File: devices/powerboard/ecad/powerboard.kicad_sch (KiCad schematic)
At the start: 42 parts, among them J1 Conn_02x02_Top_Bottom, J10 Conn_02x01, J2 Conn_02x02_Top_Bottom, J3 Conn_02x01, J4 Conn_02x01, J5 USB_A, J6 JST PH, J7 JST PH, J8 47053-1000, J9 USB_A, Q2 MMBT3904, U1 TPS51386RJNR, U2 EMC2101-ACZL

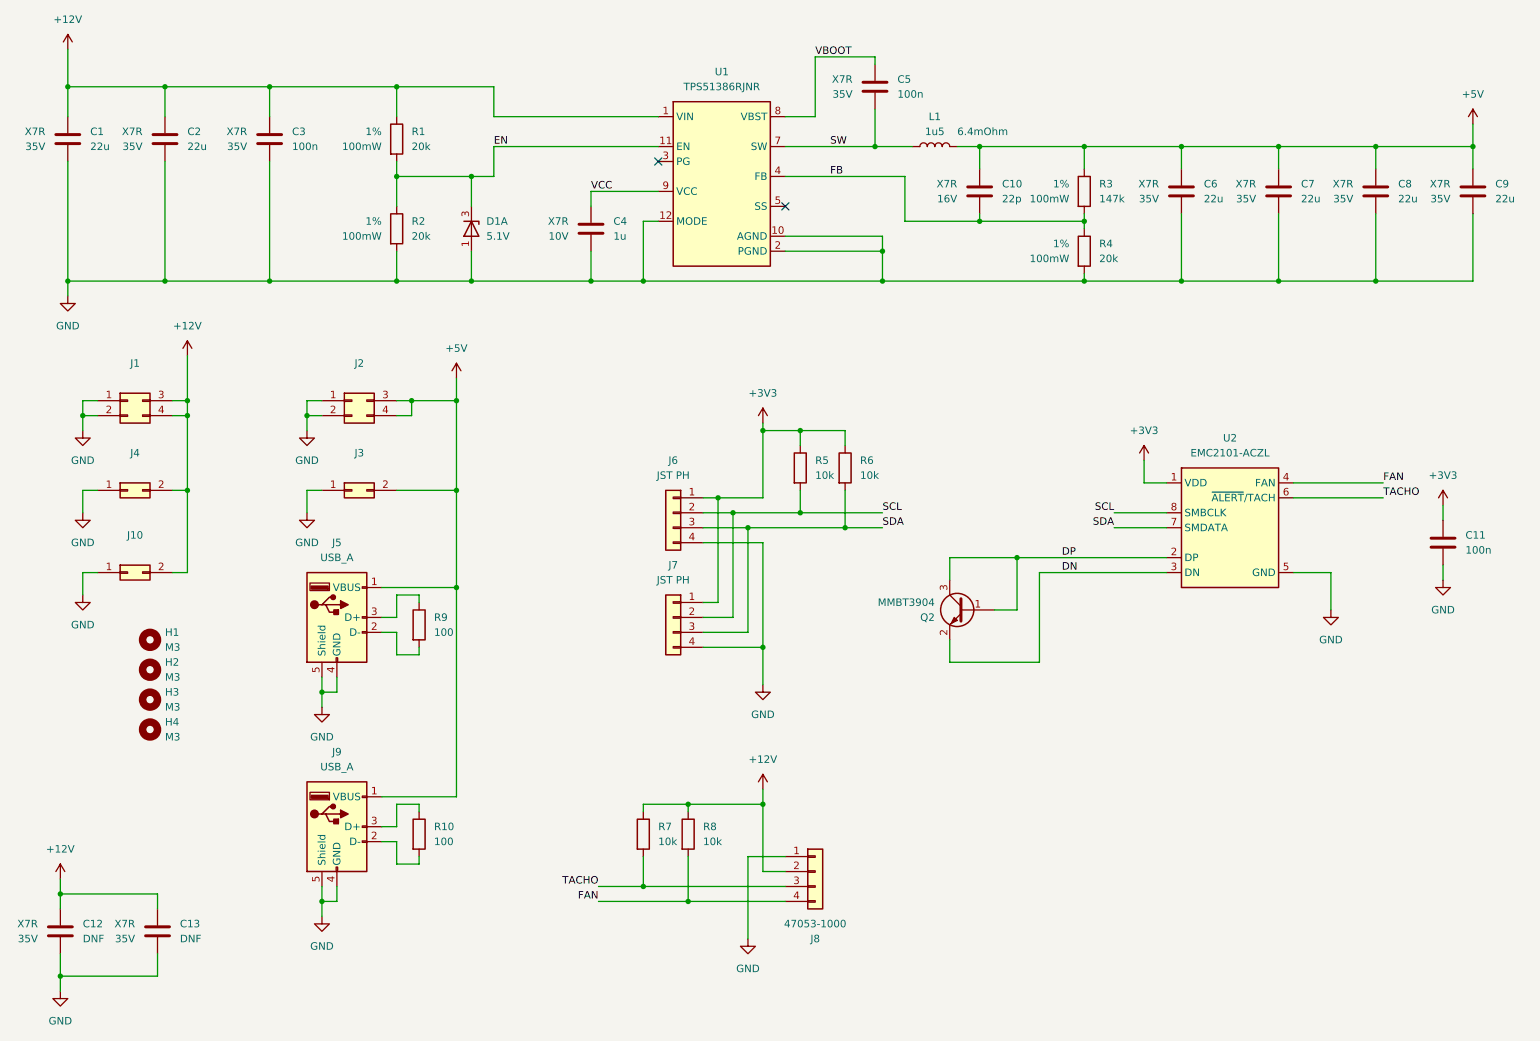
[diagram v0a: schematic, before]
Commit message: Powerboard revA done
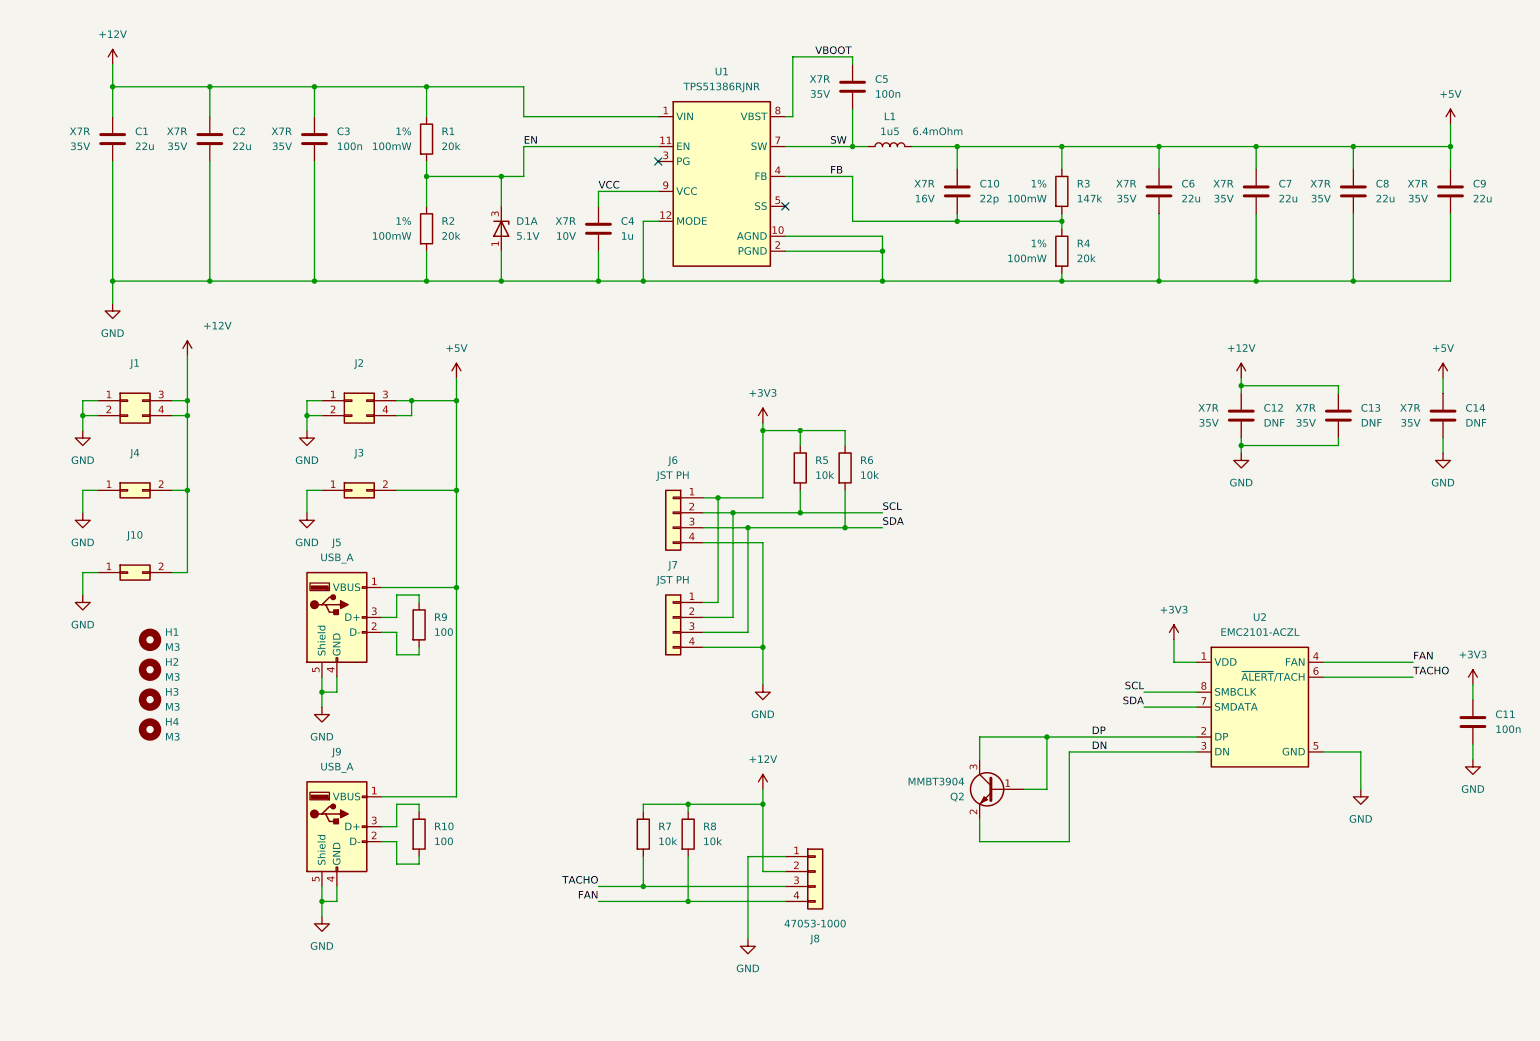
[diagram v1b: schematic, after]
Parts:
- added C14: DNF, Capacitor_SMD:C_0603_1608Metric, symbol Device:C
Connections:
- net +5V: now also C14.1
- net GND: now also C14.2
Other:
- moved on the sheet: C1, C10, C11, C2, C3, C4, C5, C6, C7, C8, C9, D1A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
